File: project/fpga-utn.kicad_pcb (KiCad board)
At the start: 2 copper layers, 148 parts, among them J1 USB_C_Receptacle_USB2.0_16P, P1 Conector SMD 2x10, P2 Conector SMD 2x10, P3 Conector SMD 2x10, P4 Conector SMD 2x10, SW1 SW_Push, SW2 SW_Push, SW3 SW_Push, SW4 SW_Push, SW5 SW_Push, SW6 SW_Push, SW7 SW_Push, SW8 SW_Push, U1 LD1117S33TR_SOT223, U2 LD1117S12TR_SOT223, U3 USBLC6-2SC6, U4 FT2232HL, U5 M93C66, U6 ICE40HX4K-TQ144, U7 W25X40CLSN, Y1 ECS-3225MV-120-CN-TR, Y2 ECS-3225MVQ-1000-CN-TR

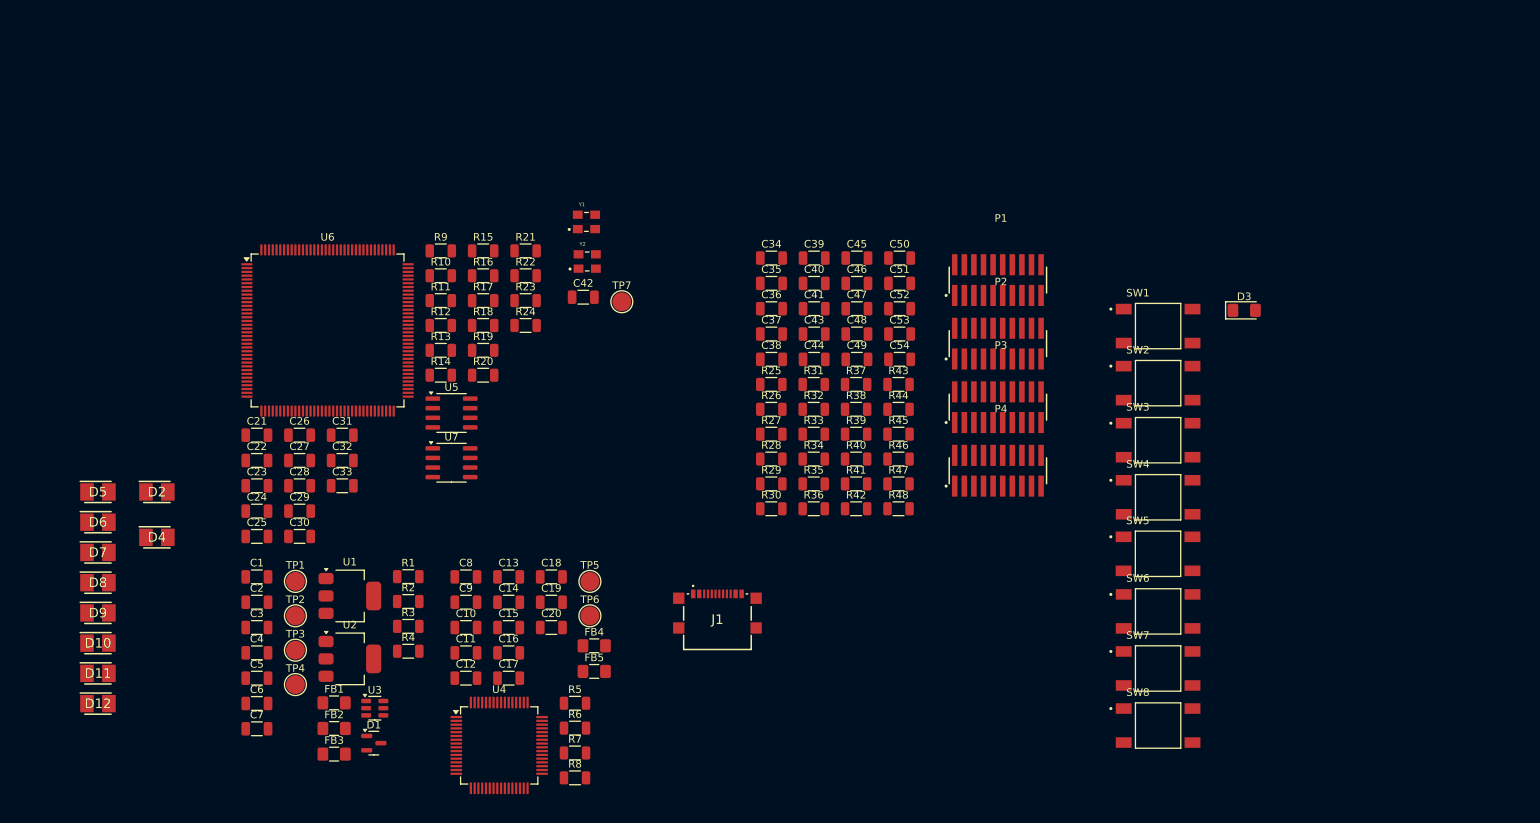
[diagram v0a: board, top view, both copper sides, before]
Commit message: PCB etapa de potencia y comunicacion lista
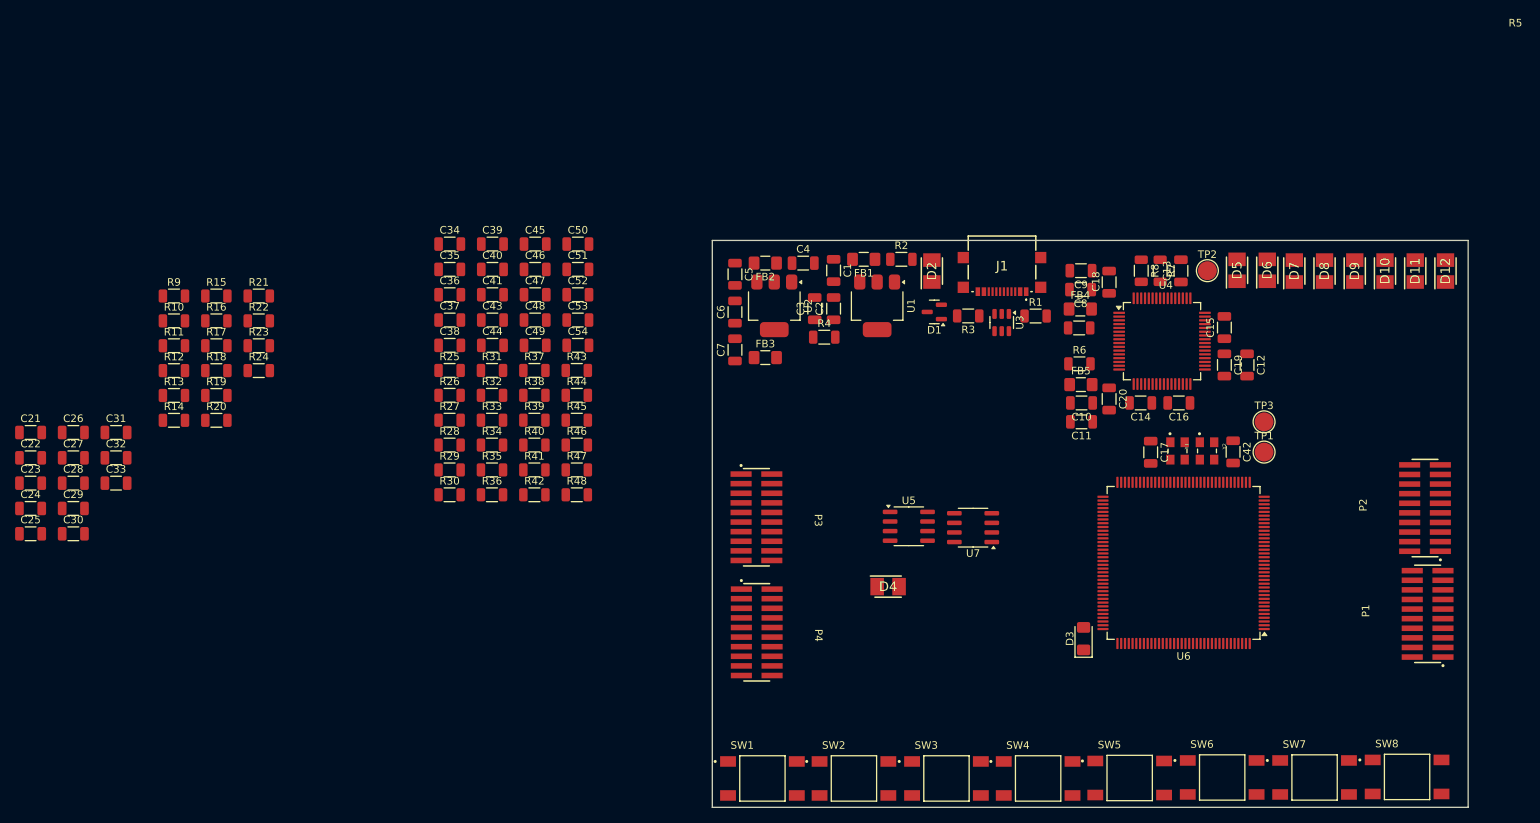
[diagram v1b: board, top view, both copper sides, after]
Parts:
- removed the TP1 at (84.3, 92.6)
- removed the TP2 at (84.3, 97.2)
- removed the TP3 at (84.3, 101.7)
- removed TP4: TP4_GND, TestPoint:TestPoint_Pad_D2.5mm
- moved D12 187.2 mm to (236.5, 51.5), turned to 90 degrees
- moved D11 182.2 mm to (232.5, 51.5), turned to 90 degrees
- moved D10 177.3 mm to (228.5, 51.5), turned to 90 degrees
- moved D9 172.3 mm to (224.5, 51.5), turned to 90 degrees
- moved D8 167.4 mm to (220.5, 51.5), turned to 90 degrees
- moved D7 162.6 mm to (216.5, 51.5), turned to 90 degrees
- moved D6 158.3 mm to (212.9, 51.5), turned to 90 degrees
- moved D5 153.5 mm to (208.9, 51.5), turned to 90 degrees
- moved U6 117.4 mm to (201.8, 90.2), turned to 180 degrees
- moved C12 111.3 mm to (210.2, 64.0), turned to -90 degrees
- moved D2 106.6 mm to (168.6, 51.5), turned to 90 degrees
- moved U4 102.7 mm to (199.0, 60.8)
- moved C15 102.7 mm to (207.2, 59.0), turned to 90 degrees
- moved R8 100.6 mm to (196.2, 51.5), turned to -90 degrees
- moved R7 100.3 mm to (198.8, 51.5), turned to -90 degrees
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- renumbered TP6 to TP1, TP5 to TP2, TP7 to TP3
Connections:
- U6 pad 110: /Perifericos/LED1 -> unconnected-(U6A-IOT_168-Pad110)
- U6 pad 112: /Perifericos/LED2 -> unconnected-(U6A-IOT_169-Pad112)
- U6 pad 113: /Perifericos/LED3 -> unconnected-(U6A-IOT_170-Pad113)
- U6 pad 114: /Perifericos/LED4 -> unconnected-(U6A-IOT_171-Pad114)
- U6 pad 115: /Perifericos/LED5 -> unconnected-(U6A-IOT_172-Pad115)
- U6 pad 116: /Perifericos/LED6 -> unconnected-(U6A-IOT_173-Pad116)
- U6 pad 117: /Perifericos/LED7 -> unconnected-(U6A-IOT_174-Pad117)
- U6 pad 118: /Perifericos/LED8 -> unconnected-(U6A-IOT_177-Pad118)
- U6 pad 37: unconnected-(U6C-IOB_56-Pad37) -> /Perifericos/LED1
- U6 pad 38: unconnected-(U6C-IOB_57-Pad38) -> /Perifericos/LED2
- U6 pad 39: unconnected-(U6C-IOB_61-Pad39) -> /Perifericos/LED3
- U6 pad 41: unconnected-(U6C-IOB_63-Pad41) -> /Perifericos/LED4
- U6 pad 42: unconnected-(U6C-IOB_64-Pad42) -> /Perifericos/LED5
- U6 pad 43: unconnected-(U6C-IOB_71-Pad43) -> /Perifericos/LED6
- U6 pad 44: unconnected-(U6C-IOB_72-Pad44) -> /Perifericos/LED7
- U6 pad 45: unconnected-(U6C-IOB_73-Pad45) -> /Perifericos/LED8
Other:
- board outline added: 100 x 75 mm
